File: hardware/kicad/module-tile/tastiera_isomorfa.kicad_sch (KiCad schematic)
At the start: 4 parts, among them J1 Conn_LEFT, J2 Conn_TOP, J3 Conn_BOTTOM, J4 Conn_RIGHT

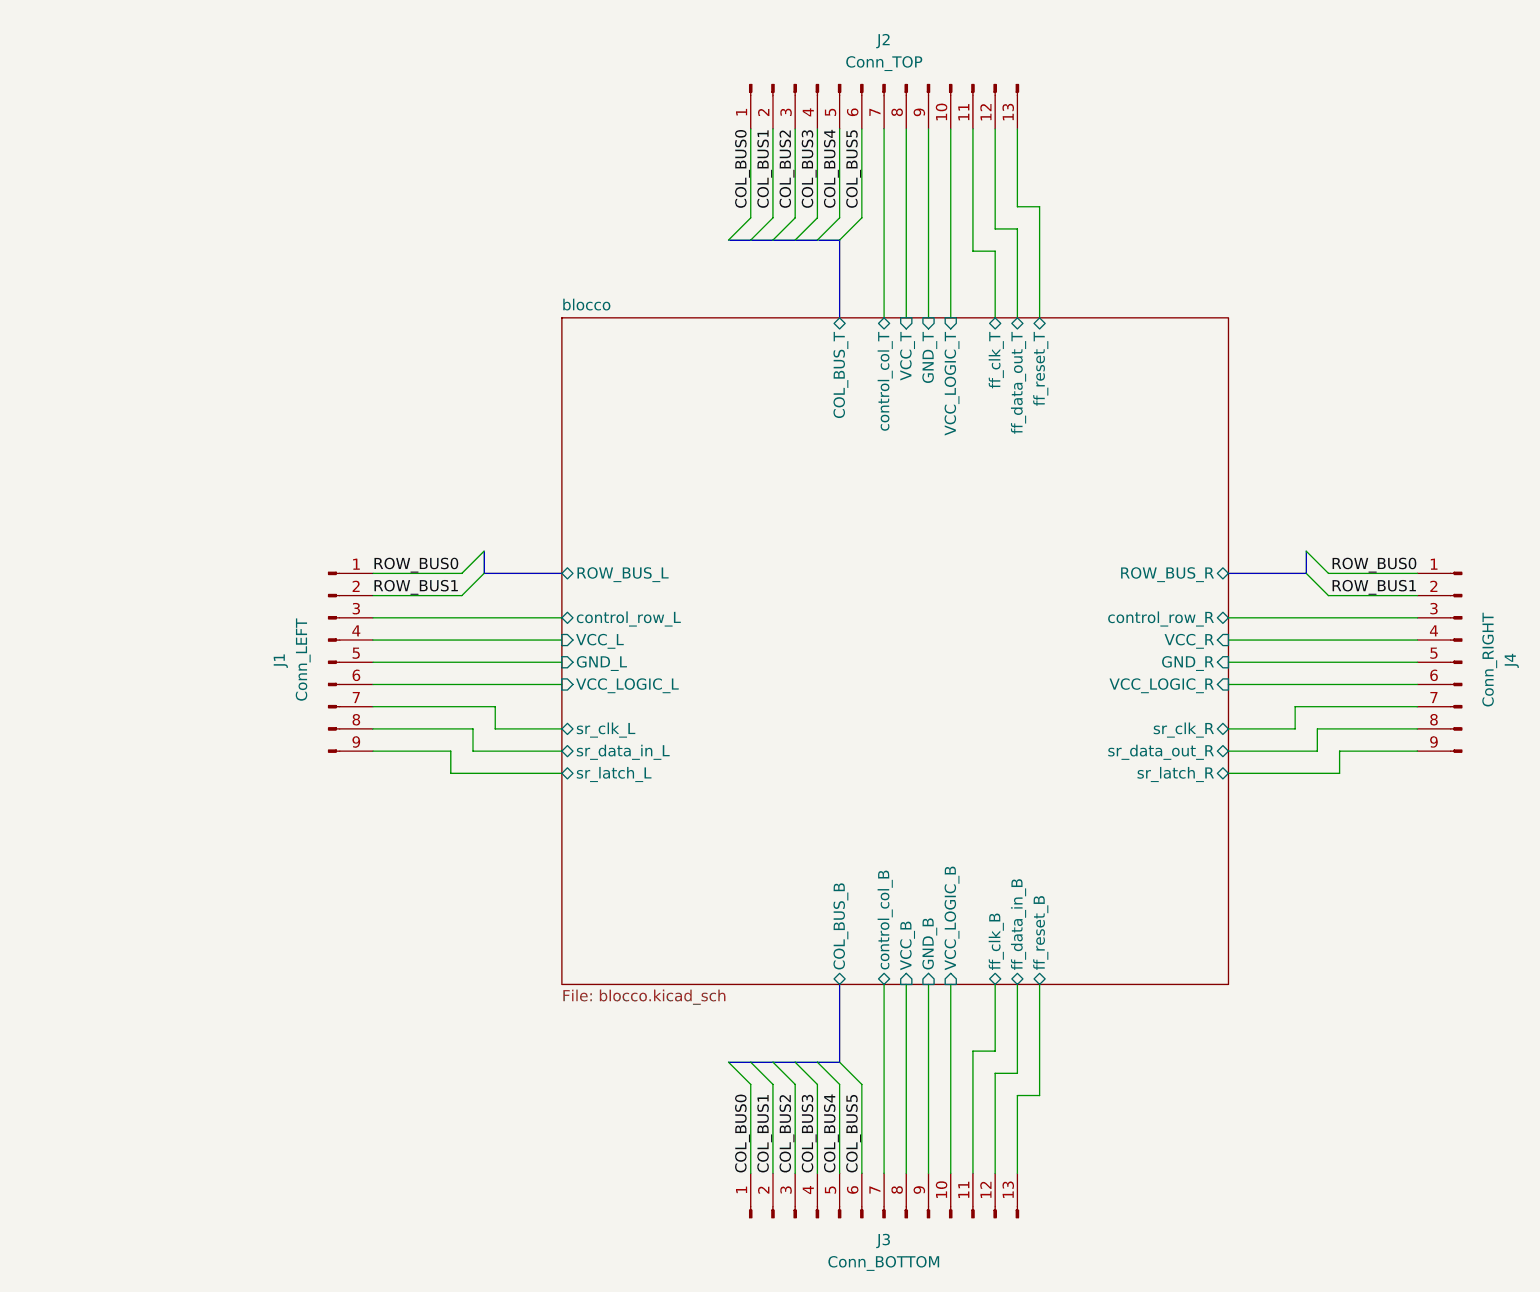
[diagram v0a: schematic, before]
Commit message: starting new topology
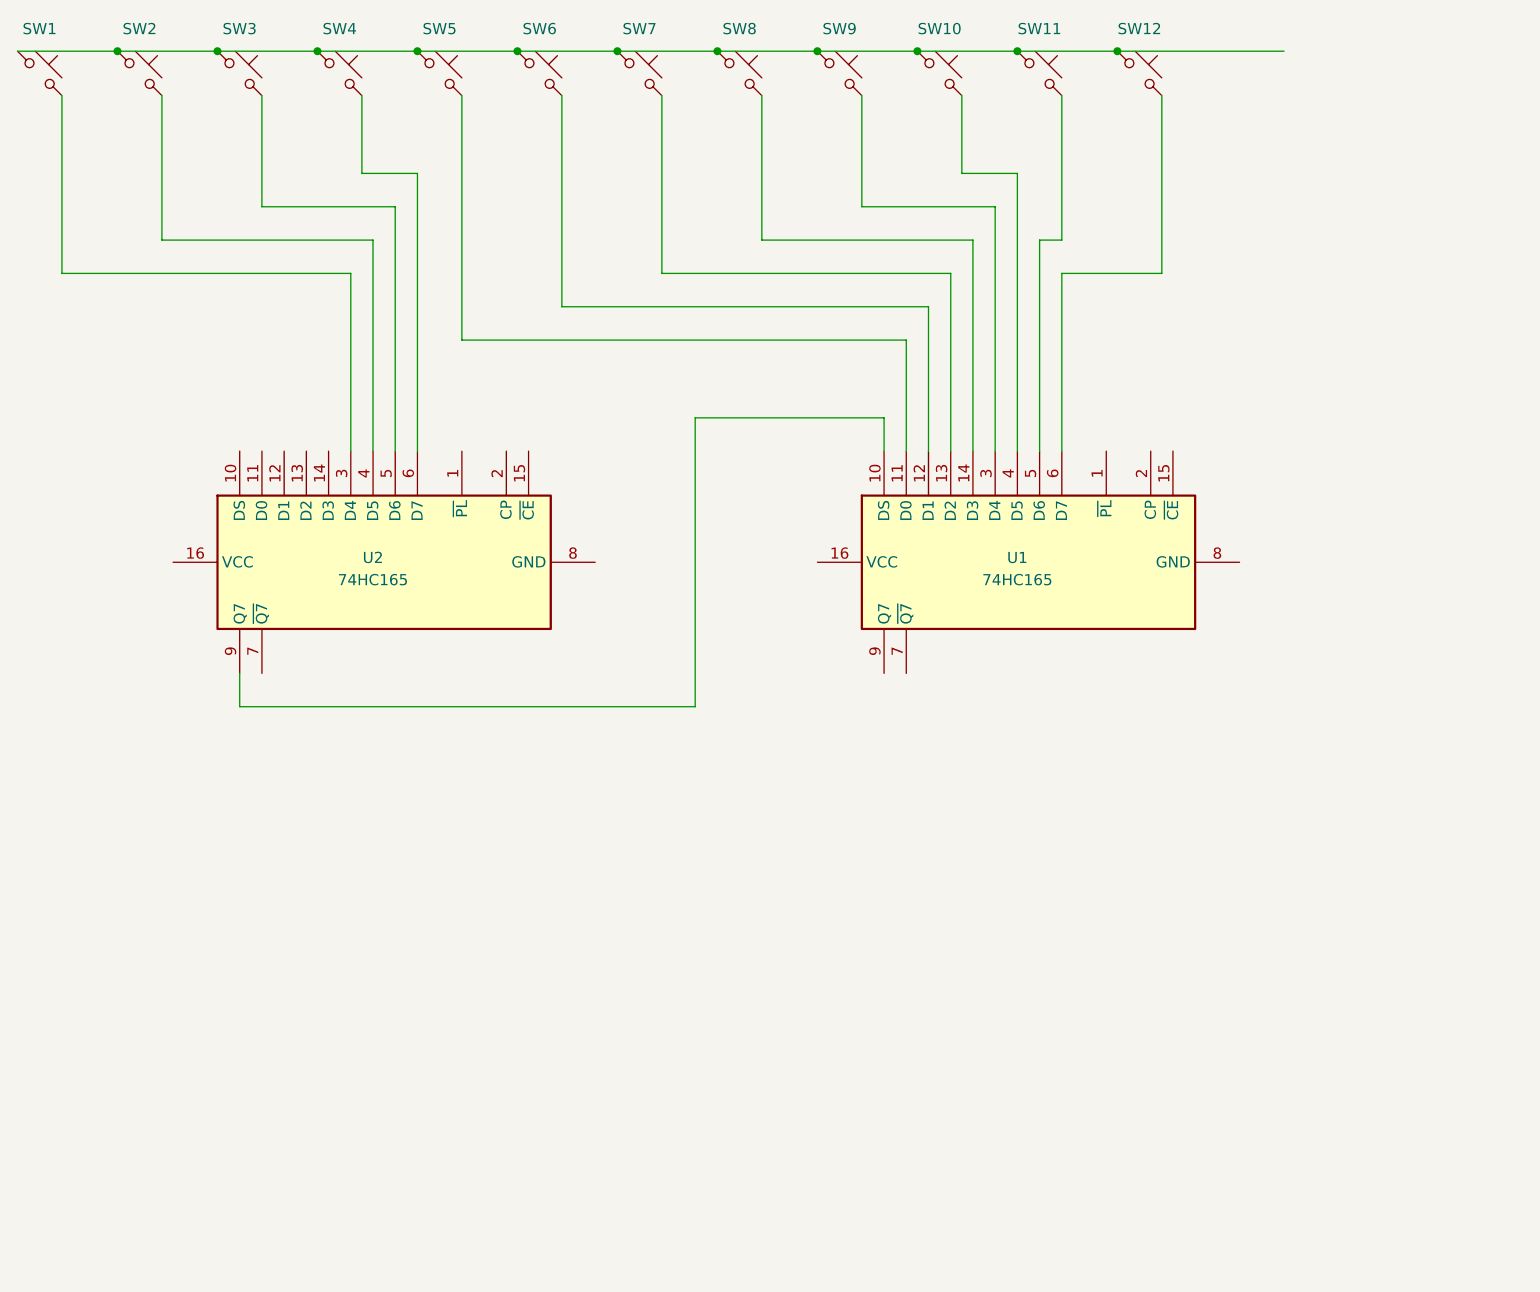
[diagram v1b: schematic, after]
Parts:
- removed J1: Conn_LEFT, symbol Connector:Conn_01x09_Pin
- removed J2: Conn_TOP, symbol Connector:Conn_01x13_Pin
- removed J3: Conn_BOTTOM, symbol Connector:Conn_01x13_Pin
- removed J4: Conn_RIGHT, symbol Connector:Conn_01x09_Pin
- added SW1, SW10, SW11, SW12, SW2, SW3, SW4, SW5, SW6, SW7, SW8, SW9: ~, symbol Switch:SW_Push_45deg
- added U1, U2: 74HC165, symbol 74xx:74HC165
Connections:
- new net: SW1.1, SW10.1, SW11.1, SW12.1, SW2.1, SW3.1, SW4.1, SW5.1, SW6.1, SW7.1, SW8.1, SW9.1
- new net: SW12.2, U1.6 (D7)
- new net: SW8.2, U1.14 (D3)
- new net: U1.10 (DS), U2.9 (Q7)
- new net: SW5.2, U1.11 (D0)
- new net: SW6.2, U1.12 (D1)
- new net: SW7.2, U1.13 (D2)
- new net: SW9.2, U1.3 (D4)
- new net: SW10.2, U1.4 (D5)
- new net: SW11.2, U1.5 (D6)
- new net: SW4.2, U2.6 (D7)
- new net: SW2.2, U2.4 (D5)
- new net: SW1.2, U2.3 (D4)
- new net: SW3.2, U2.5 (D6)
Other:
- removed sheet blocco
